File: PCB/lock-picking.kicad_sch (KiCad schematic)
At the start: 22 parts, among them U1 HX PZ2.54-1X5P ZZ, U2 DRV8876PWPR, U3 MLX90393SLW-ABA-011-RE, U4 SMTSOM225BTR, U5 S2B-PH-K-S, U6 SMTSOM225BTR, U7 HX TYPE-C 16PIN, U8 AMS1117-5.0_C347223

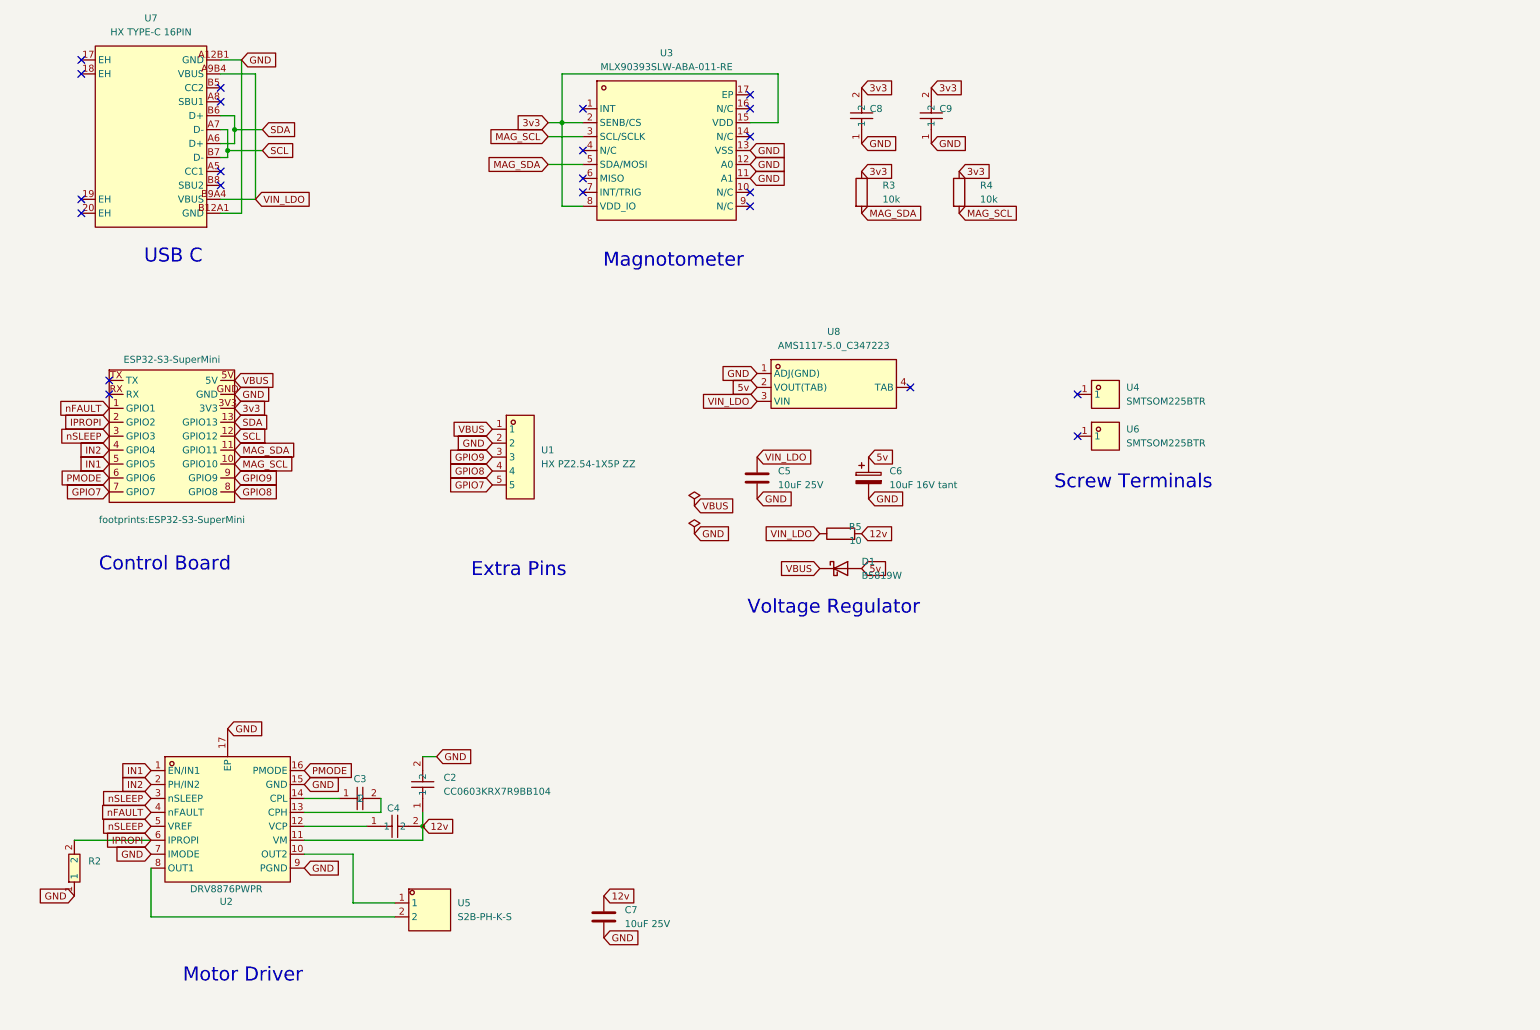
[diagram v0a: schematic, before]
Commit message: schematic claude edit
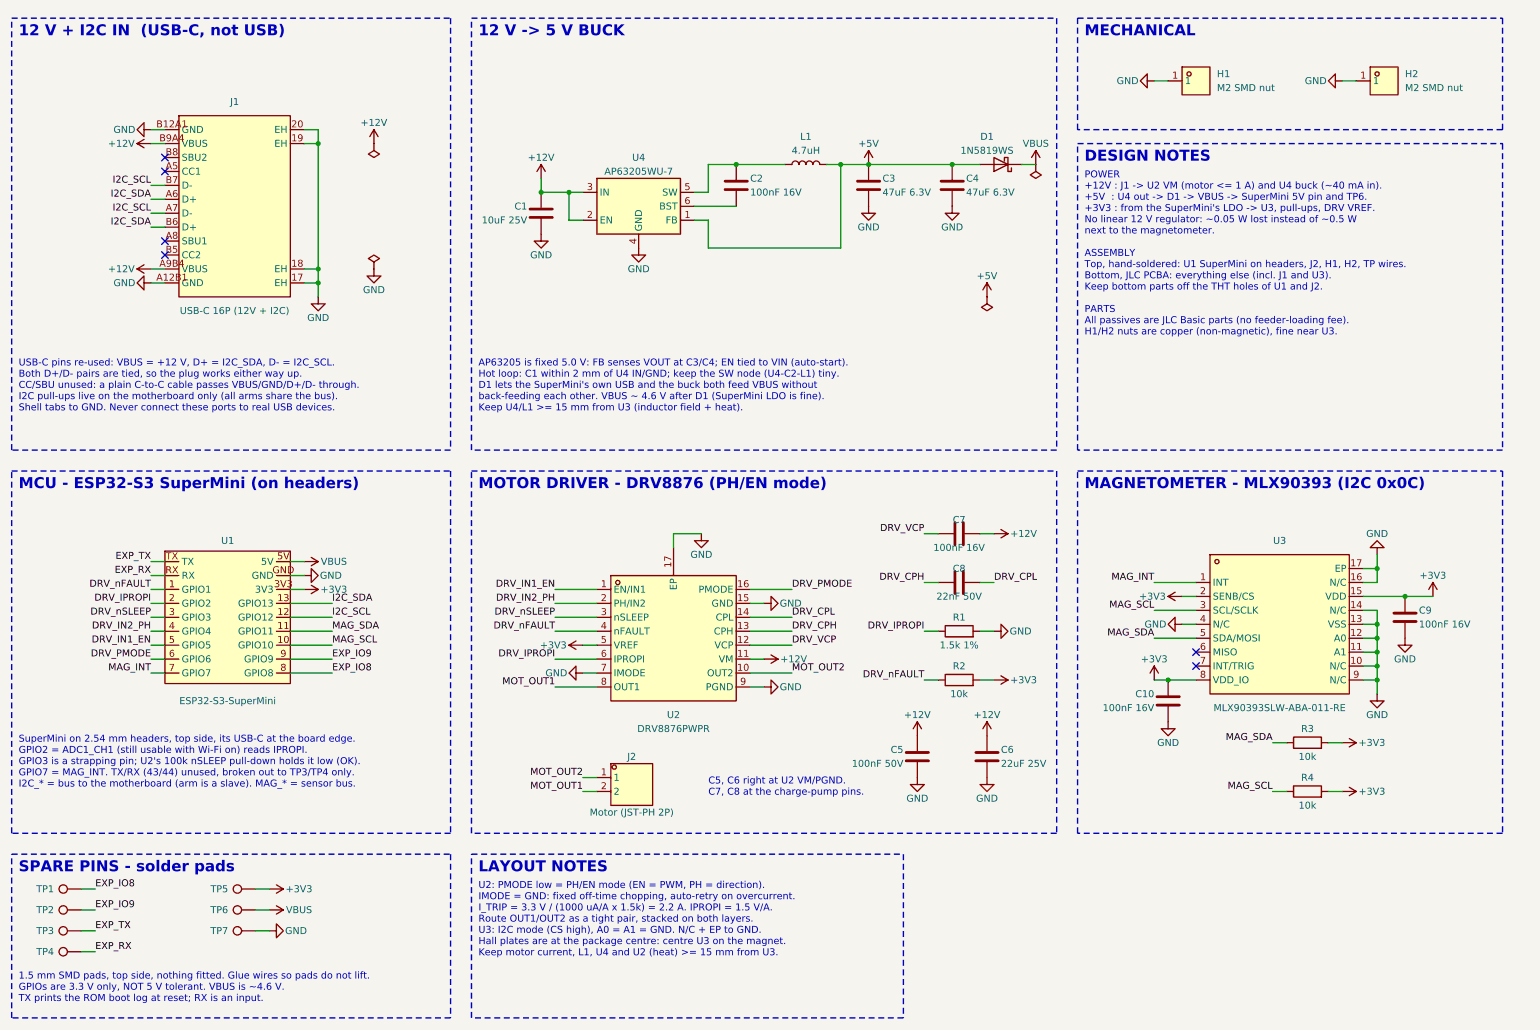
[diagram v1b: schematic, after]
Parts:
- removed C6: 10uF 16V tant, Capacitor_Tantalum_SMD:CP_EIA-3216-18_Kemet-A, symbol Device:C_Polarized
- removed R5: 10, Resistor_SMD:R_0805_2012Metric, symbol Device:R
- removed U1: HX PZ2.54-1X5P ZZ, EasyEDA:HDR-TH_5P-P2.54-V-M, symbol EasyEDA:HXPZ2.54-1X5PZZ
- removed U8: AMS1117-5.0_C347223, EasyEDA:SOT-223_L6.7-W3.5-P2.30-BR, symbol EasyEDA:AMS1117-5.0_C347223
- added C2: 100nF 16V, Capacitor_SMD:C_0402_1005Metric, symbol Device:C
- added C3, C4: 47uF 6.3V, Capacitor_SMD:C_0805_2012Metric, symbol Device:C
- added L1: 4.7uH, Inductor_SMD:L_Changjiang_FTC252012S, symbol Device:L
- added R2: 10k, Resistor_SMD:R_0402_1005Metric, symbol Device:R
- added TP1, TP2, TP3, TP4, TP5, TP6, TP7: Pad, TestPoint:TestPoint_Pad_D1.5mm, symbol Connector:TestPoint
- added U4: AP63205WU-7, Package_TO_SOT_SMD:TSOT-23-6, symbol Regulator_Switching:AP63205WU
- C1: renamed from C5; Manufacturer Samsung -> Samsung Electro-Mechanics
- C10: renamed from C8; value CC0603KRX7R9BB104 -> 100nF 16V; footprint EasyEDA:C0603 -> Capacitor_SMD:C_0402_1005Metric; symbol EasyEDA:CC0603KRX7R9BB104 -> Device:C; LCSC Part C14663 -> C1525; MPN CC0603KRX7R9BB104 -> CL05B104KO5NNNC; Manufacturer YAGEO -> Samsung Electro-Mechanics
- C5: renamed from C2; value CC0603KRX7R9BB104 -> 100nF 50V; footprint EasyEDA:C0603 -> Capacitor_SMD:C_0402_1005Metric; symbol EasyEDA:CC0603KRX7R9BB104 -> Device:C; LCSC Part C14663 -> C307331; MPN CC0603KRX7R9BB104 -> CL05B104KB54PNC; Manufacturer YAGEO(国巨) -> Samsung Electro-Mechanics
- C6: renamed from C7; value 10uF 25V -> 22uF 25V; footprint Capacitor_SMD:C_0805_2012Metric -> Capacitor_SMD:C_1206_3216Metric; LCSC Part C15850 -> C12891; MPN CL21A106KAYNNNE -> CL31A226KAHNNNE; Manufacturer Samsung -> Samsung Electro-Mechanics
- C7: renamed from C4; value CC0603KRX7R9BB104 -> 100nF 16V; footprint EasyEDA:C0603 -> Capacitor_SMD:C_0402_1005Metric; symbol EasyEDA:CC0603KRX7R9BB104 -> Device:C; LCSC Part C14663 -> C1525; MPN CC0603KRX7R9BB104 -> CL05B104KO5NNNC; Manufacturer YAGEO(国巨) -> Samsung Electro-Mechanics
- C8: renamed from C3; value CL10B223KB8NNNC-22nF -> 22nF 50V; footprint EasyEDA:C0603 -> Capacitor_SMD:C_0402_1005Metric; symbol EasyEDA:CL10B223KB8NNNC -> Device:C; LCSC Part C21122 -> C1532; MPN CL10B223KB8NNNC -> 0402B223K500NT; Manufacturer SAMSUNG(三星) -> FH (Guangdong Fenghua)
- C9: value CC0603KRX7R9BB104 -> 100nF 16V; footprint EasyEDA:C0603 -> Capacitor_SMD:C_0402_1005Metric; symbol EasyEDA:CC0603KRX7R9BB104 -> Device:C; LCSC Part C14663 -> C1525; MPN CC0603KRX7R9BB104 -> CL05B104KO5NNNC; Manufacturer YAGEO -> Samsung Electro-Mechanics
- D1: value B5819W -> 1N5819WS; footprint Diode_SMD:D_SOD-123 -> Diode_SMD:D_SOD-323; LCSC Part C8598 -> C191023; MPN B5819W SL -> 1N5819WS; Manufacturer JSCJ -> Guangdong Hottech
- H1: renamed from U4; value SMTSOM225BTR -> M2 SMD nut
- H2: renamed from U6; value SMTSOM225BTR -> M2 SMD nut
- J1: renamed from U7; value HX TYPE-C 16PIN -> USB-C 16P (12V + I2C)
- J2: renamed from U5; value S2B-PH-K-S -> Motor (JST-PH 2P)
- R1: renamed from R2; value 0603WAF1501T5E -> 1.5k 1%; footprint EasyEDA:R0603 -> Resistor_SMD:R_0402_1005Metric; symbol EasyEDA:0603WAF1501T5E -> Device:R; LCSC Part C22843 -> C25867; MPN 0603WAF1501T5E -> 0402WGF1501TCE; Manufacturer UNI-ROYAL(厚声) -> UNI-ROYAL
- R3, R4: footprint EasyEDA:R0603 -> Resistor_SMD:R_0402_1005Metric; LCSC Part C25804 -> C25744; MPN 0603WAF1002T5E -> 0402WGF1002TCE
- renumbered ESP1 to U1
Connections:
- net GPIO7 is gone; now on net MAG_INT: U1.7 (GPIO7)
- net VIN_LDO is gone; now on net +12V: C1.1, J1.A9B4 (VBUS), J1.B9A4 (VBUS)
- net GND: now also C10.2, C9.2, H1.1, H2.1, J1.17 (EH), J1.18 (EH), J1.19 (EH), J1.20 (EH), R1.2, U3.10 (N/C), U3.14 (N/C), U3.16 (N/C), U3.17 (EP), U3.4 (N/C), U3.9 (N/C), C3.2, C4.2, TP7.1, U4.4 (GND); no longer C10.1, C9.1, R1.1
- net MAG_SCL: now also R4.1; no longer R4.2
- net MAG_SDA: now also R3.1; no longer R3.2
- net VBUS: now also TP6.1
- net DRV_VCP: now reaches C7.1, U2.12 (VCP)
- net EXP_RX: now reaches U1.RX
- net EXP_RX: now also TP4.1
- net EXP_TX: now reaches U1.TX
- net EXP_TX: now also TP3.1
- net MAG_INT: now reaches U3.1 (INT)
- net DRV_CPH: now reaches C8.1
- net DRV_CPH: now also U2.13 (CPH); no longer U2.14 (CPL)
- net DRV_CPL: now reaches C8.2
- net DRV_CPL: now also U2.14 (CPL); no longer U2.13 (CPH)
- net MOT_OUT2: now reaches J2.1, U2.10 (OUT2)
- net MOT_OUT1: now reaches J2.2, U2.8 (OUT1)
- net 12v renamed +12V
- net +12V: now also U4.2 (EN), U4.3 (IN)
- net 3v3 renamed +3V3
- net +3V3: now also C10.1, C9.1, R3.2, R4.2, U2.5 (VREF), R2.2, TP5.1; no longer C10.2, C9.2, R3.1, R4.1
- net 5v renamed +5V
- net +5V: now also C3.1, C4.1, L1.2, U4.1 (FB)
- net GPIO8 renamed EXP_IO8
- net EXP_IO8: now also TP1.1
- net GPIO9 renamed EXP_IO9
- net EXP_IO9: now also TP2.1
- net IN1 renamed DRV_IN1_EN
- net IN2 renamed DRV_IN2_PH
- net IPROPI renamed DRV_IPROPI
- net DRV_IPROPI: now also R1.1; no longer R1.2
- net PMODE renamed DRV_PMODE
- net SCL renamed I2C_SCL
- net SDA renamed I2C_SDA
- net nFAULT renamed DRV_nFAULT
- net DRV_nFAULT: now also R2.1
- net nSLEEP renamed DRV_nSLEEP
- net DRV_nSLEEP: no longer U2.5 (VREF)
- new net: C2.1, L1.1, U4.5 (SW)
- new net: C2.2, U4.6 (BST)
- no-connect marks 22 -> 6
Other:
- note added: "1.5 mm SMD pads, top side, nothing fitted. Glue wires so pads do not lift. GPIOs are 3.3 V only, NOT 5 V tolerant. VBUS is ~4.6 V. TX prints the ROM boot log at reset; RX is an input."
- note added: "12 V + I2C IN (USB-C, not USB)"
- note added: "12 V -> 5 V BUCK"
- note added: "AP63205 is fixed 5.0 V: FB senses VOUT at C3/C4; EN tied to VIN (auto-start). Hot loop: C1 within 2 mm of U4 IN/GND; keep the SW node (U4-C2-L1) tiny. D1 lets the SuperMini's own USB and the buck both feed VBUS without back-feeding each other. VBUS ~ 4.6 V after D1 (SuperMini LDO is fine). Keep U4/L1 >= 15 mm from U3 (inductor field + heat)."
- note added: "C5, C6 right at U2 VM/PGND. C7, C8 at the charge-pump pins."
- note added: "DESIGN NOTES"
- note added: "LAYOUT NOTES"
- note added: "MAGNETOMETER - MLX90393 (I2C 0x0C)"
- note added: "MCU - ESP32-S3 SuperMini (on headers)"
- note added: "MECHANICAL"
- note added: "MOTOR DRIVER - DRV8876 (PH/EN mode)"
- note added: "POWER +12V : J1 -> U2 VM (motor <= 1 A) and U4 buck (~40 mA in). +5V : U4 out -> D1 -> VBUS -> SuperMini 5V pin and TP6. +3V3 : from the SuperMini's LDO -> U3, pull-ups, DRV VREF. No linear 12 V regulator: ~0.05 W lost instead of ~0.5 W next to the magnetometer. ASSEMBLY Top, hand-soldered: U1 SuperMini on headers, J2, H1, H2, TP wires. Bottom, JLC PCBA: everything else (incl. J1 and U3). Keep bo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"
- note added: "SPARE PINS - solder pads"
- note added: "SuperMini on 2.54 mm headers, top side, its USB-C at the board edge. GPIO2 = ADC1_CH1 (still usable with Wi-Fi on) reads IPROPI. GPIO3 is a strapping pin; U2's 100k nSLEEP pull-down holds it low (OK). GPIO7 = MAG_INT. TX/RX (43/44) unused, broken out to TP3/TP4 only. I2C_* = bus to the motherboard (arm is a slave). MAG_* = sensor bus."
- note added: "U2: PMODE low = PH/EN mode (EN = PWM, PH = direction). IMODE = GND: fixed off-time chopping, auto-retry on overcurrent. I_TRIP = 3.3 V / (1000 uA/A x 1.5k) = 2.2 A. IPROPI = 1.5 V/A. Route OUT1/OUT2 as a tight pair, stacked on both layers. U3: I2C mode (CS high), A0 = A1 = GND. N/C + EP to GND. Hall plates are at the package centre: centre U3 on the magnet. Keep motor current, L1, U4 and U2 (heat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"
- note added: "USB-C pins re-used: VBUS = +12 V, D+ = I2C_SDA, D- = I2C_SCL. Both D+/D- pairs are tied, so the plug works either way up. CC/SBU unused: a plain C-to-C cable passes VBUS/GND/D+/D- through. I2C pull-ups live on the motherboard only (all arms share the bus). Shell tabs to GND. Never connect these ports to real USB devices."
- note removed: "Control Board"
- note removed: "Extra Pins"
- note removed: "Magnotometer"
- note removed: "Motor Driver"
- note removed: "Screw Terminals"
- note removed: "USB C"
- note removed: "Voltage Regulator"
- title: Lock Picking Robot -> Lock Picking Robot - Arm Board
- moved on the sheet: C1, C6, D1, H1, H2, J1, J2, R3, R4, U2, U3
